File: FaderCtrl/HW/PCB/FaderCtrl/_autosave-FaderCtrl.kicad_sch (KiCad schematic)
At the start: 89 parts, among them J1 PDI, J2 Barrel_Jack_MountingPin, J3 PWM, J4 PORTD, J5 MPS, J6 MPP, J7 MPN, P1 USB_C_Plug_USB2.0, U1 ATxmega256A3BU-A, U2 TSR_1-2450, U3 AMS1117-3.3, Y1 32k

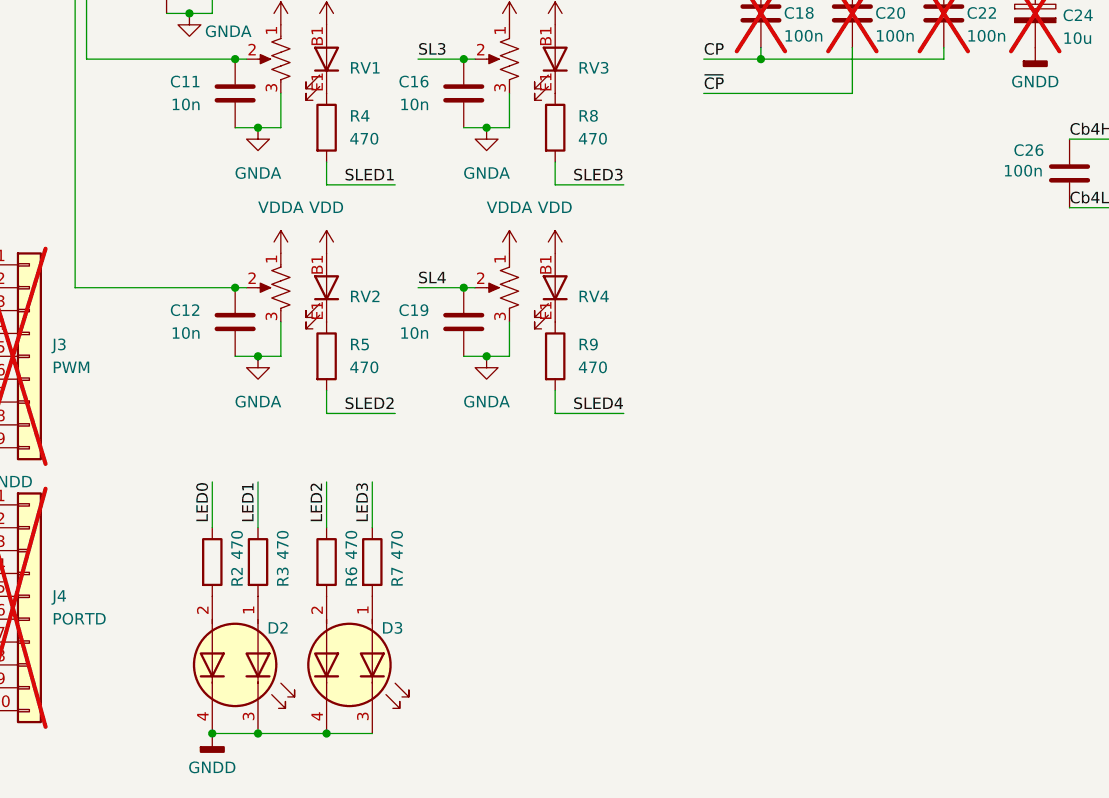
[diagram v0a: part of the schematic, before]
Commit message: a
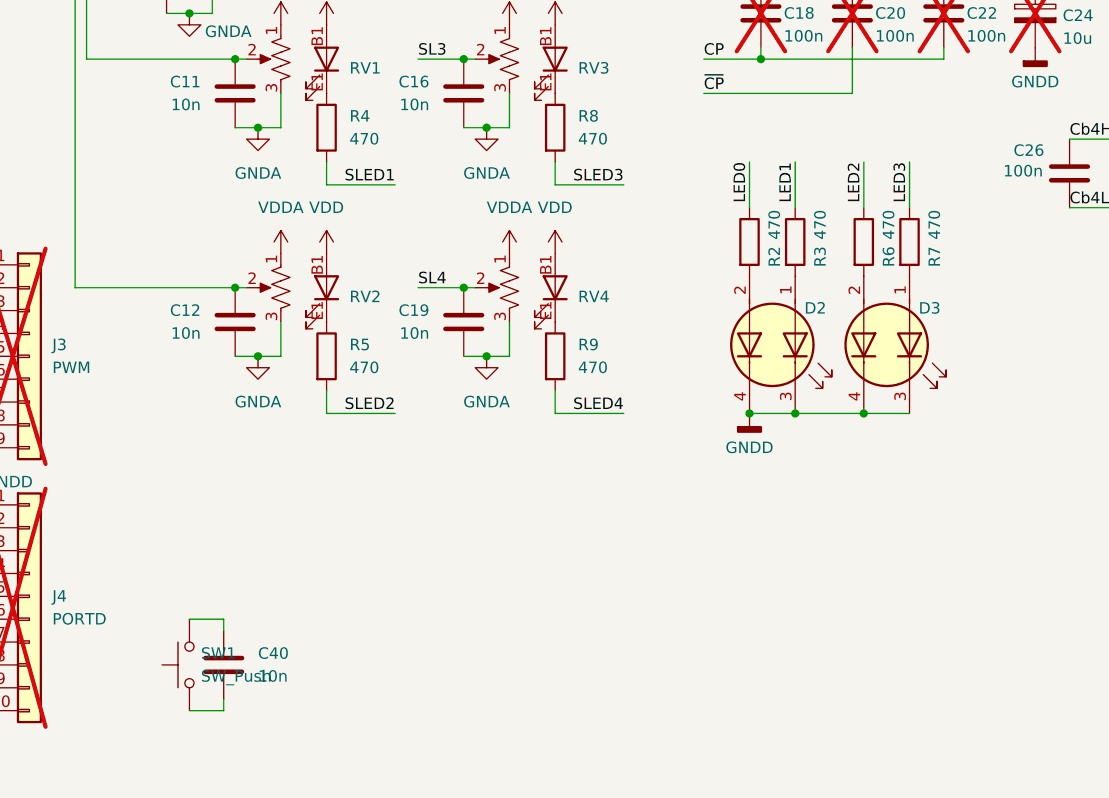
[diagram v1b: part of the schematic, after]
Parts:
- added C40: 10n, Capacitor_SMD:C_0603_1608Metric_Pad1.08x0.95mm_HandSolder, symbol Device:C
- added SW1: SW_Push, symbol Switch:SW_Push
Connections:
- new net: C40.2, SW1.1
- new net: C40.1, SW1.2
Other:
- moved on the sheet: D2, D3, R2, R3, R6, R7
